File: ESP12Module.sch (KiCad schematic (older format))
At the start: 19 parts, among them J1 Conn_01x05_Male, J2 Conn_01x05_Male, J3 Screw_Terminal_01x02, J4 Conn_01x02_Male, SW4 SW_Push, U2 ESP-12S, sw3 SW_Push

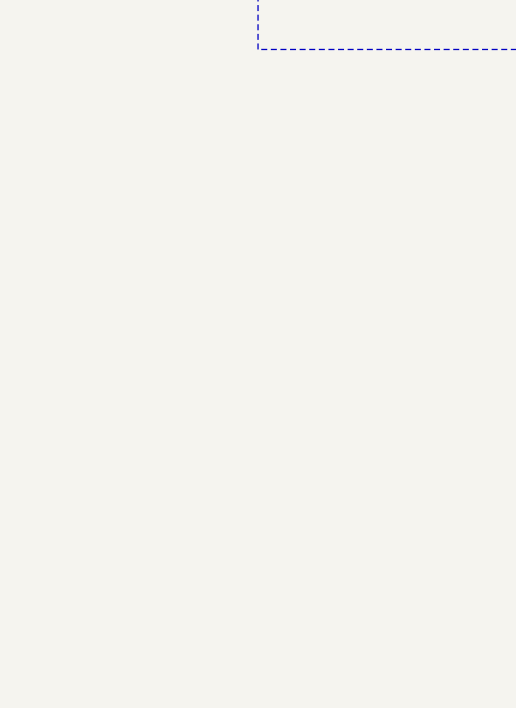
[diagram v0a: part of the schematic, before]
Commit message: Added amp
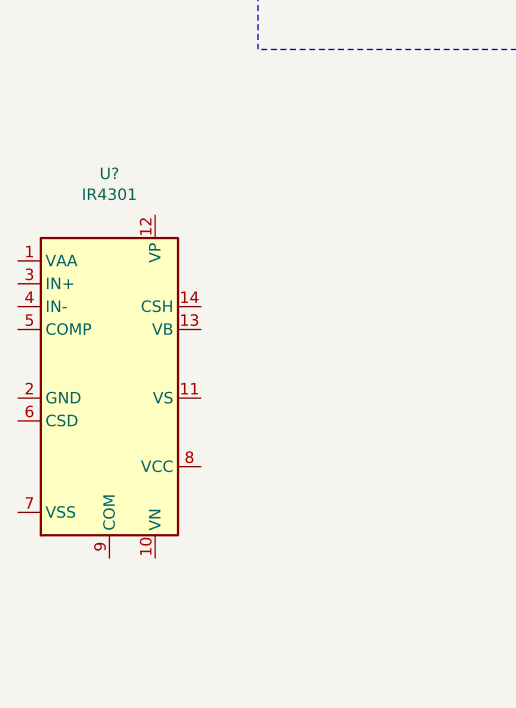
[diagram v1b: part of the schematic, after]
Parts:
- added U?: IR4301, Package_DFN_QFN:Infineon_PQFN-22-15-4EP_6x5mm_P0.65mm, symbol Amplifier_Audio:IR4301
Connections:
- new net: U?.15 (COM), U?.9 (COM)
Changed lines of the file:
@@
 	7950 3750 7950 3850
 Connection ~ 7950 3850
+$Comp
+L Amplifier_Audio:IR4301 U?
+U 1 1 5F6871D4
+P 3450 3675
+F 0 "U?" H 3450 4656 50  0000 C CNN
+F 1 "IR4301" H 3450 4565 50  0000 C CNN
+F 2 "Package_DFN_QFN:Infineon_PQFN-22-15-4EP_6x5mm_P0.65mm" H 3450 3675 50  0001 C CIN
+F 3 "https://www.infineon.com/dgdl/ir4301.pdf?fileId=5546d462533600a4015355d5fc691819" H 3450 3675 50  0001 C CNN
+	1    3450 3675
+	1    0    0    -1
+$EndComp
 $EndSCHEMATC
